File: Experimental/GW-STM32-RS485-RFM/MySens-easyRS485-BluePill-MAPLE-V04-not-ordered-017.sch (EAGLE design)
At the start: 40 parts, among them IC2 LAN-USR-ES1, IC5 LD117ADT50TR, IC6 LM1117MPX-ADJ, U1 RFM69HCW, U2 RFM69HCW, X3 1751264

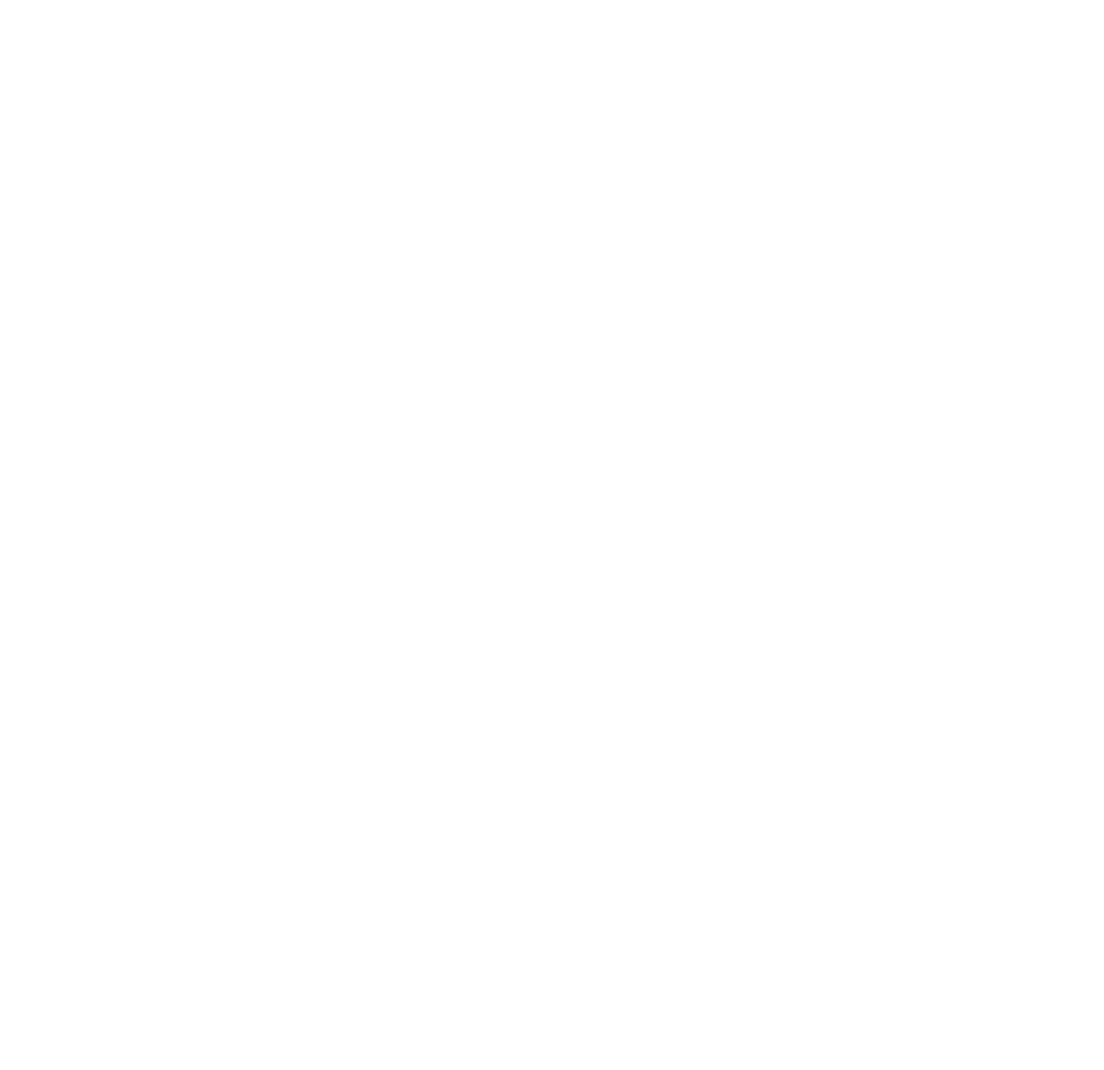
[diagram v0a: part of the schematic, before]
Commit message: stm32 update
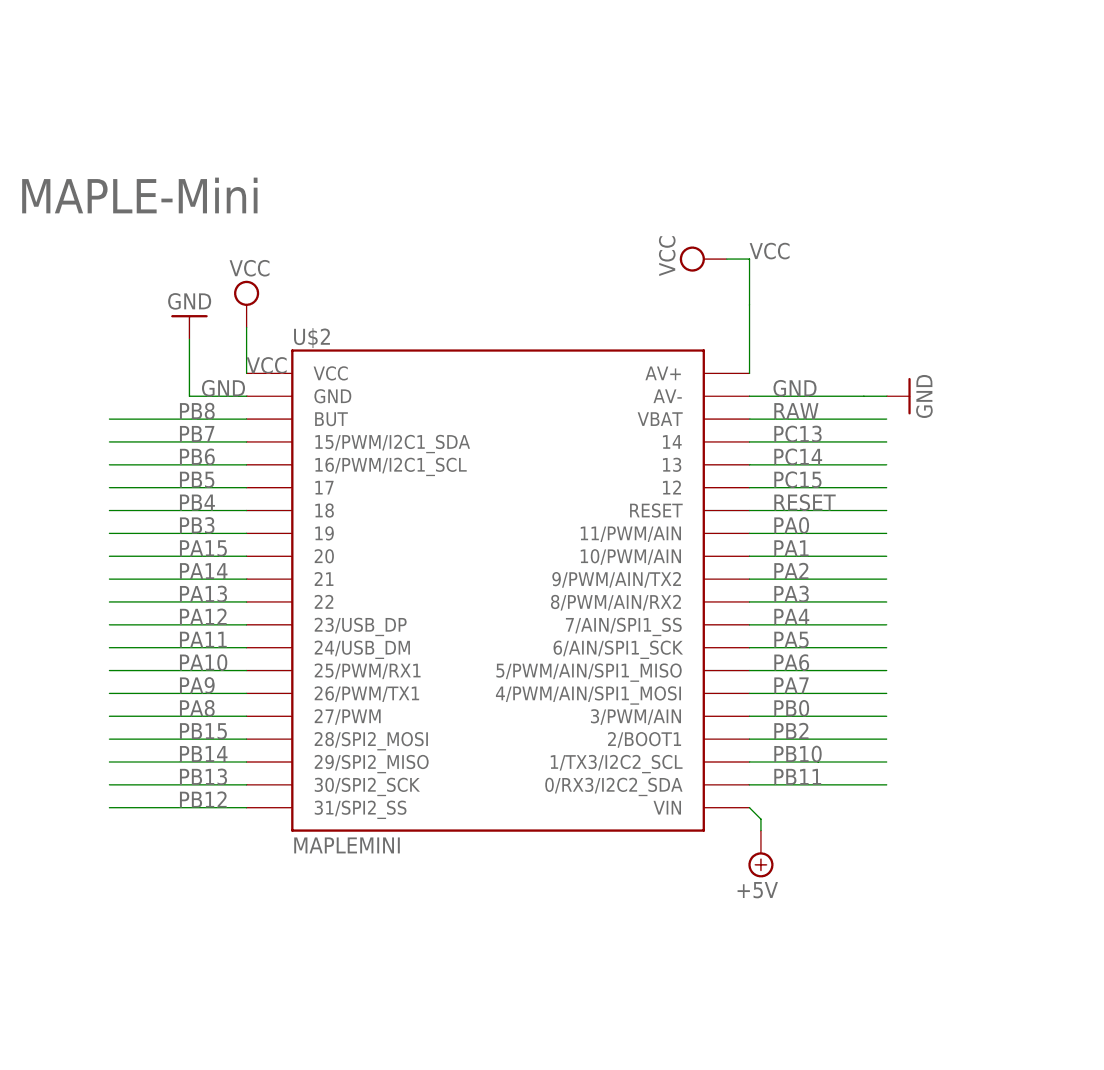
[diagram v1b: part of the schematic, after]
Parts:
- added U$2: MAPLEMINI, maplemini-small:MAPLEMINI
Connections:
- new net +5V: U$2.VIN
- new net PA13: U$2.22
- new net PA14: U$2.21
- new net PB2: U$2.2/BOOT1
- new net RAW: U$2.VBAT
- net GND: now also U$2.AV-, U$2.GND
- net PA0: now also U$2.11/PWM/AIN
- net PA1: now also U$2.10/PWM/AIN
- net PA10: now also U$2.25/PWM/RX1
- net PA11: now also U$2.24/USB_DM
- net PA12: now also U$2.23/USB_DP
- net PA15: now also U$2.20
- net PA2: now also U$2.9/PWM/AIN/TX2
- net PA3: now also U$2.8/PWM/AIN/RX2
- net PA4: now also U$2.7/AIN/SPI1_SS
- net PA5: now also U$2.6/AIN/SPI1_SCK
- net PA6: now also U$2.5/PWM/AIN/SPI1_MISO
- net PA7: now also U$2.4/PWM/AIN/SPI1_MOSI
- net PA8: now also U$2.27/PWM
- net PA9: now also U$2.26/PWM/TX1
- net PB0: now also U$2.3/PWM/AIN
- net PB10: now also U$2.1/TX3/I2C2_SCL
- net PB11: now also U$2.0/RX3/I2C2_SDA
- net PB12: now also U$2.31/SPI2_SS
- net PB13: now also U$2.30/SPI2_SCK
- net PB14: now also U$2.29/SPI2_MISO
- net PB15: now also U$2.28/SPI2_MOSI
- net PB3: now also U$2.19
- net PB4: now also U$2.18
- net PB5: now also U$2.17
- net PB6: now also U$2.16/PWM/I2C1_SCL
- net PB7: now also U$2.15/PWM/I2C1_SDA
- net PB8: now also U$2.BUT
- net PC13: now also U$2.14
- net PC14: now also U$2.13
- net PC15: now also U$2.12
- net RESET: now also U$2.RESET
- net VCC: now also U$2.AV+, U$2.VCC
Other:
- note added: "MAPLE-Mini"
